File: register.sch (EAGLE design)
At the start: 28 parts, among them IC1 74AS574N, IC2 74AS574N, IC3 74AC283N, IC4 74AC283N, IC5 74AC283N, IC6 74AC283N, IC7 74AC244N, IC8 74AC244N

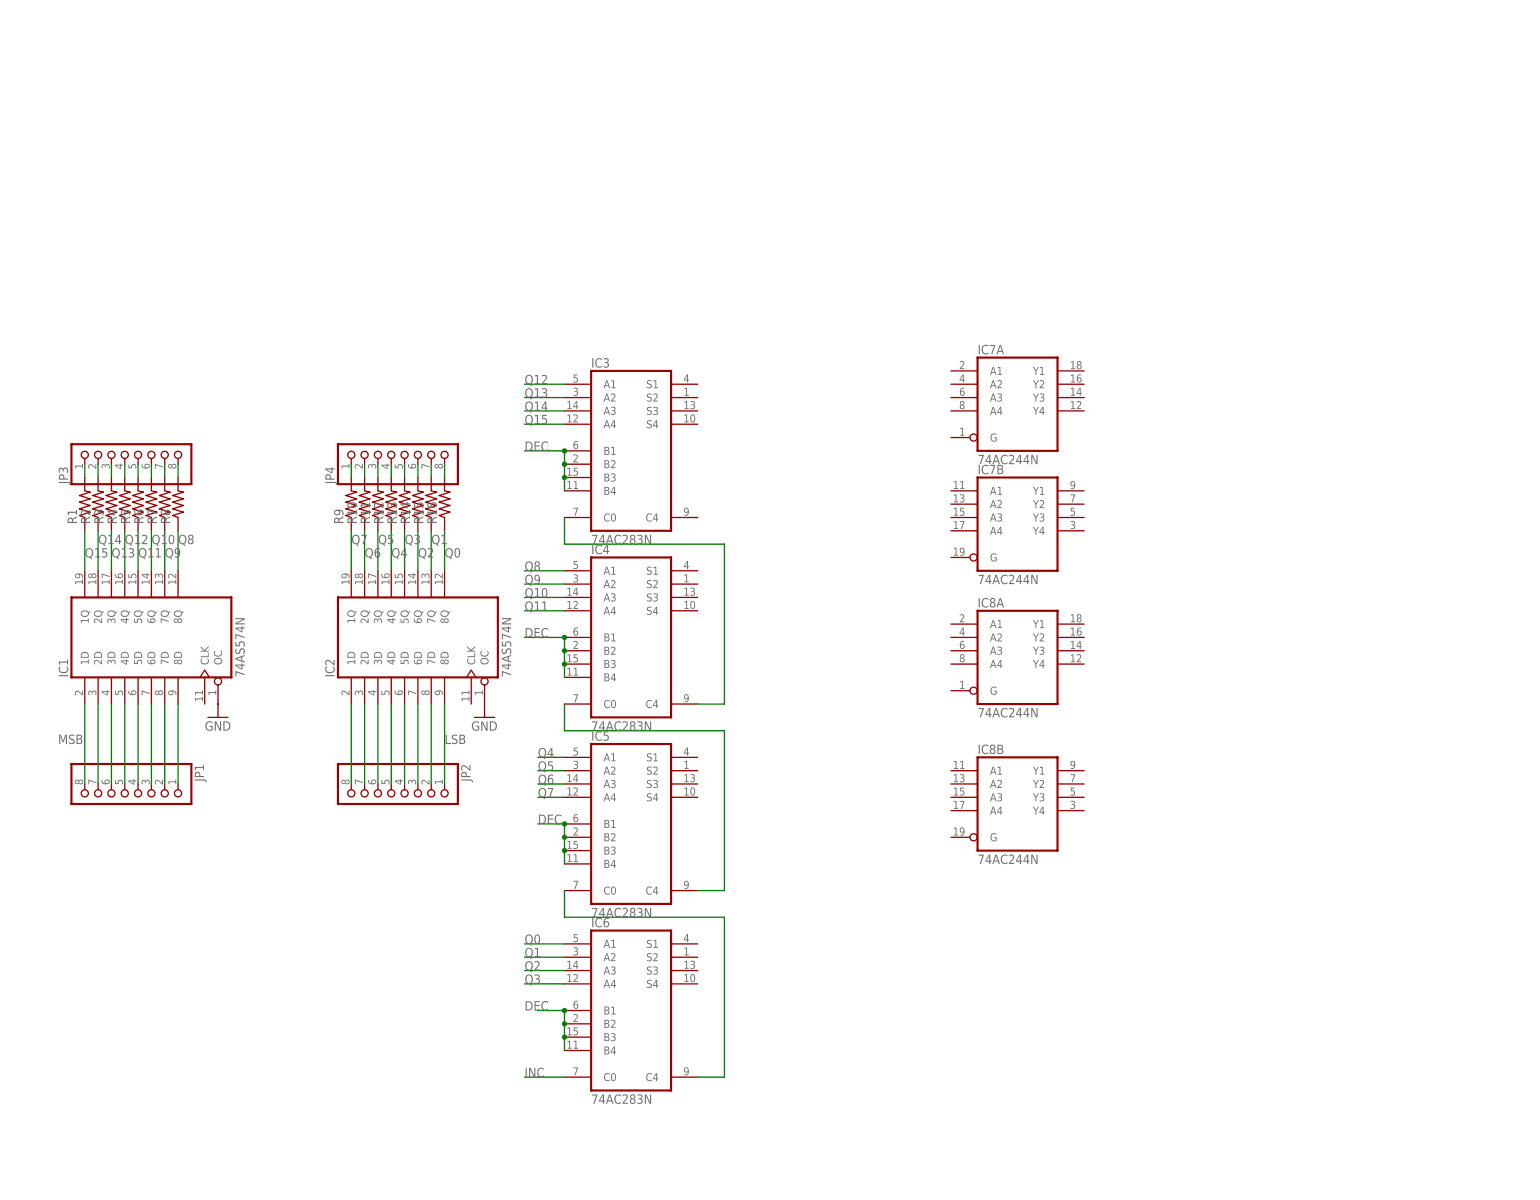
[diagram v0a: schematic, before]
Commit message: some work
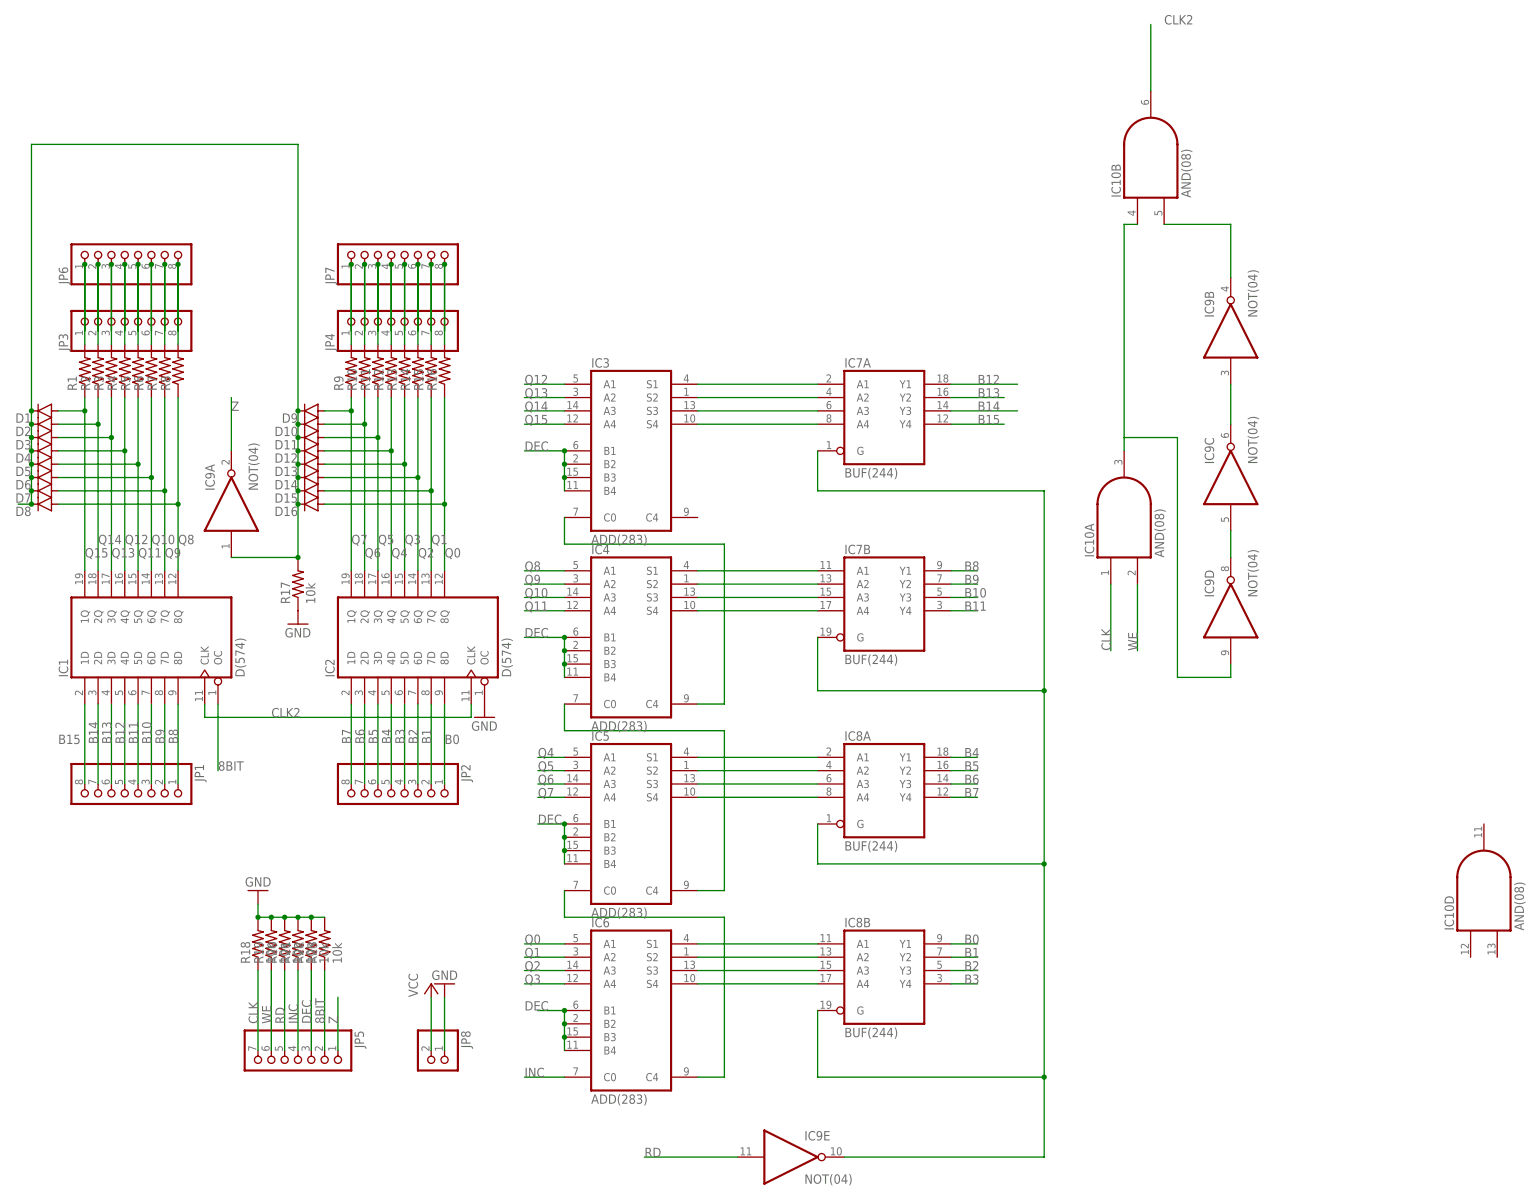
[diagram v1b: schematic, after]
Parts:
- added D1, D10, D11, D12, D13, D14, D15, D16, D2, D3, D4, D5, D6, D7, D8, D9: (no value), diode:DIODE-D-7.5
- added IC10: AND(08), 74xx-us:74ALS08N
- added IC9: NOT(04), 74xx-us:74ALS04N
- added JP5: (no value), pinhead:PINHD-1X7
- added JP6, JP7: (no value), pinhead:PINHD-1X8
- added JP8: (no value), pinhead:PINHD-1X2
- added R17, R18, R19, R20, R21, R22, R23: 10k, rcl:R-US_0204/7
- IC1, IC2: value 74AS574N -> D(574); MOUSER (none) -> 595-SN74HCT574NE4
- IC3, IC4, IC5, IC6: value 74AC283N -> ADD(283); MOUSER (none) -> 595-CD74HCT283E
- IC7, IC8: value 74AC244N -> BUF(244); MOUSER (none) -> 595-SN74HCT244NE4
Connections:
- removed net LSB: IC2A.8D, JP2.1
- removed net MSB: IC1A.1D, JP1.8
- removed net N$10: IC1A.7D, JP1.2
- removed net N$11: IC1A.6D, JP1.3
- removed net N$12: IC1A.5D, JP1.4
- removed net N$13: IC1A.4D, JP1.5
- removed net N$14: IC1A.3D, JP1.6
- removed net N$15: IC1A.2D, JP1.7
- removed net N$8: IC2A.1D, JP2.8
- removed net N$9: IC1A.8D, JP1.1
- new net 8BIT: IC1A.OC, JP5.2, R23.1
- new net B0: IC2A.8D, IC8B.Y1, JP2.1
- new net B1: IC2A.7D, IC8B.Y2, JP2.2
- new net B10: IC1A.6D, IC7B.Y3, JP1.3
- new net B11: IC1A.5D, IC7B.Y4, JP1.4
- new net B12: IC1A.4D, IC7A.Y1, JP1.5
- new net B13: IC1A.3D, IC7A.Y2, JP1.6
- new net B14: IC1A.2D, IC7A.Y3, JP1.7
- new net B15: IC1A.1D, IC7A.Y4, JP1.8
- new net B2: IC2A.6D, IC8B.Y3, JP2.3
- new net B3: IC2A.5D, IC8B.Y4, JP2.4
- new net B4: IC2A.4D, IC8A.Y1, JP2.5
- new net B5: IC2A.3D, IC8A.Y2, JP2.6
- new net B6: IC2A.2D, IC8A.Y3, JP2.7
- new net B7: IC2A.1D, IC8A.Y4, JP2.8
- new net B8: IC1A.8D, IC7B.Y1, JP1.1
- new net B9: IC1A.7D, IC7B.Y2, JP1.2
- new net CLK: IC10A.I0, JP5.7, R18.1
- new net CLK2: IC10B.O, IC1A.CLK, IC2A.CLK
- new net N$18: IC3A.S1, IC7A.A1
- new net N$19: IC3A.S2, IC7A.A2
- new net N$20: IC3A.S3, IC7A.A3
- new net N$21: IC3A.S4, IC7A.A4
- new net N$22: IC4A.S1, IC7B.A1
- new net N$23: IC4A.S2, IC7B.A2
- new net N$24: IC4A.S3, IC7B.A3
- new net N$25: IC4A.S4, IC7B.A4
- new net N$26: IC5A.S1, IC8A.A1
- new net N$27: IC5A.S2, IC8A.A2
- new net N$28: IC5A.S3, IC8A.A3
- new net N$29: IC5A.S4, IC8A.A4
- new net N$30: IC6A.S1, IC8B.A1
- new net N$47: IC6A.S2, IC8B.A2
- new net N$48: IC6A.S3, IC8B.A3
- new net N$49: IC6A.S4, IC8B.A4
- new net RD: IC9E.I, JP5.5, R20.1
- new net VCC: JP8.2
- new net WE: IC10A.I1, JP5.6, R19.1
- new net Z: IC9A.O, JP5.1
- net DEC: now also JP5.3, R22.1
- net GND: now also JP8.1, R17.1, R18.2, R19.2, R20.2, R21.2, R22.2, R23.2; no longer IC1A.OC
- net INC: now also JP5.4, R21.1
- net N$2: now also IC10A.O, IC10B.I0, IC9D.I; no longer IC2A.7D, JP2.2
- net N$3: now also D1.C, D10.C, D11.C, D12.C, D13.C, D14.C, D15.C, D16.C, D2.C, D3.C, D4.C, D5.C, D6.C, D7.C, D8.C, D9.C, IC9A.I, R17.2; no longer IC2A.6D, JP2.3
- net N$31: now also JP7.1
- net N$32: now also JP7.2
- net N$33: now also JP7.3
- net N$34: now also JP7.4
- net N$35: now also JP7.5
- net N$36: now also JP7.6
- net N$37: now also JP7.7
- net N$38: now also JP7.8
- net N$39: now also JP6.1
- net N$4: now also IC7A.G, IC7B.G, IC8A.G, IC8B.G, IC9E.O; no longer IC2A.5D, JP2.4
- net N$40: now also JP6.2
- net N$41: now also JP6.3
- net N$42: now also JP6.4
- net N$43: now also JP6.5
- net N$44: now also JP6.6
- net N$45: now also JP6.7
- net N$46: now also JP6.8
- net N$5: now also IC10B.I1, IC9B.O; no longer IC2A.4D, JP2.5
- net N$6: now also IC9B.I, IC9C.O; no longer IC2A.3D, JP2.6
- net N$7: now also IC9C.I, IC9D.O; no longer IC2A.2D, JP2.7
- net Q0: now also D16.A
- net Q1: now also D15.A
- net Q10: now also D6.A
- net Q11: now also D5.A
- net Q12: now also D4.A
- net Q13: now also D3.A
- net Q14: now also D2.A
- net Q15: now also D1.A
- net Q2: now also D14.A
- net Q3: now also D13.A
- net Q4: now also D12.A
- net Q5: now also D11.A
- net Q6: now also D10.A
- net Q7: now also D9.A
- net Q8: now also D8.A
- net Q9: now also D7.A
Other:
- moved on the sheet: IC7A, IC7B, IC8A, IC8B, JP3, JP4, R1, R10, R11, R12, R13, R14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
